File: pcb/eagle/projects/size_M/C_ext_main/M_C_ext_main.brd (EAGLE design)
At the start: 18 parts, among them P1 TPB1,27, U1 CP2104-F03-GM

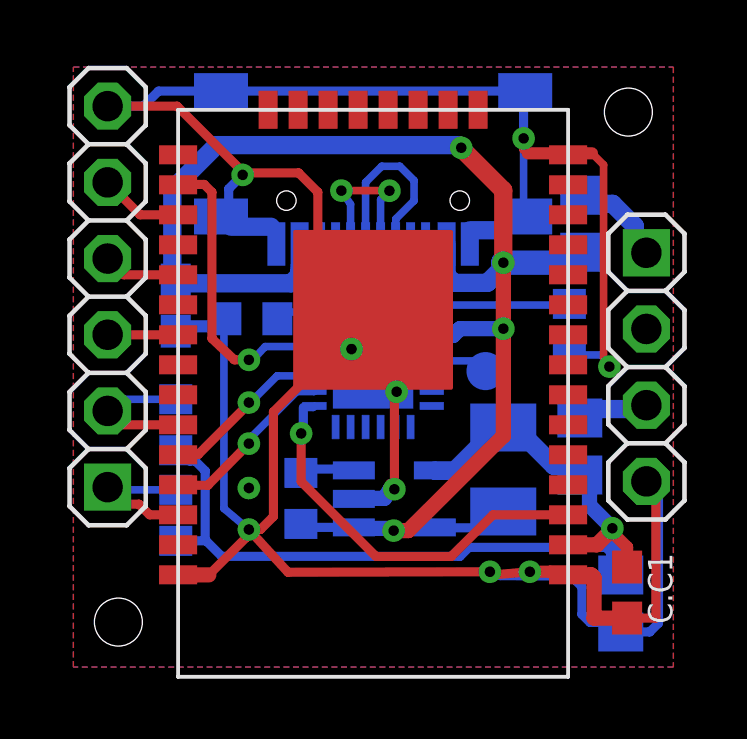
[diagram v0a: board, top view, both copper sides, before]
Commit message: PCB M.3
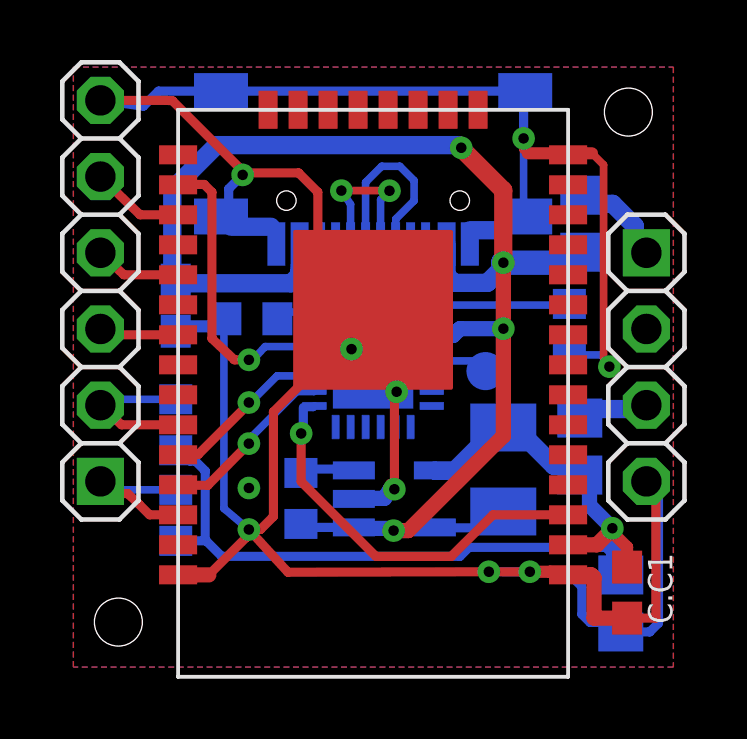
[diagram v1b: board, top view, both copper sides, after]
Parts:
- moved C.J2 0.31 mm to (1.40, 13.0)
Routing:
- net SCL: track 5.04 -> 5.66 mm
- net GND: track 127.2 -> 127.8 mm
